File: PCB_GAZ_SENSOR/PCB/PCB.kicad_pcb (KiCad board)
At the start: 2 copper layers, 68.6 x 53.3 mm, 8 parts, among them P1 Power, P2 Analog, P3 Digital, P4 Digital, P5 CONN_01X01, P6 CONN_01X01, P7 CONN_01X01, P8 CONN_01X01

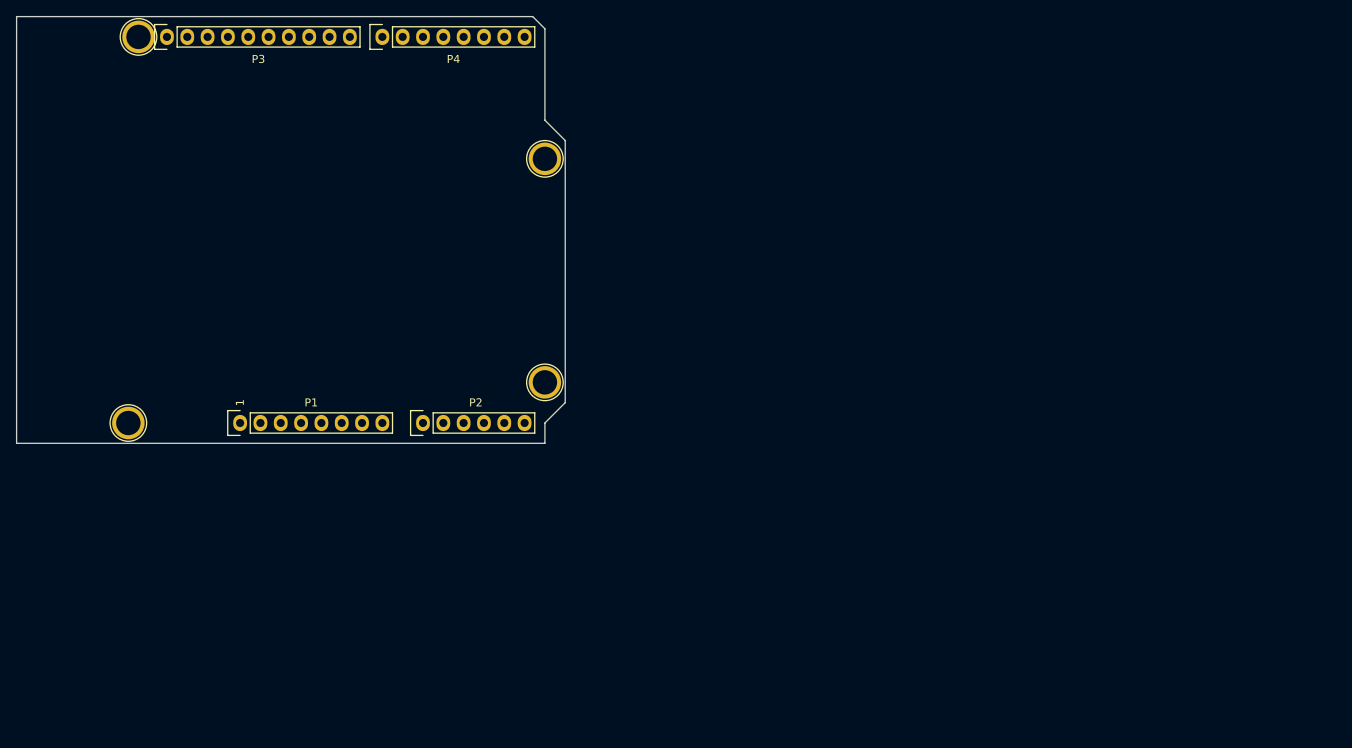
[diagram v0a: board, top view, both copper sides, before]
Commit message: final version
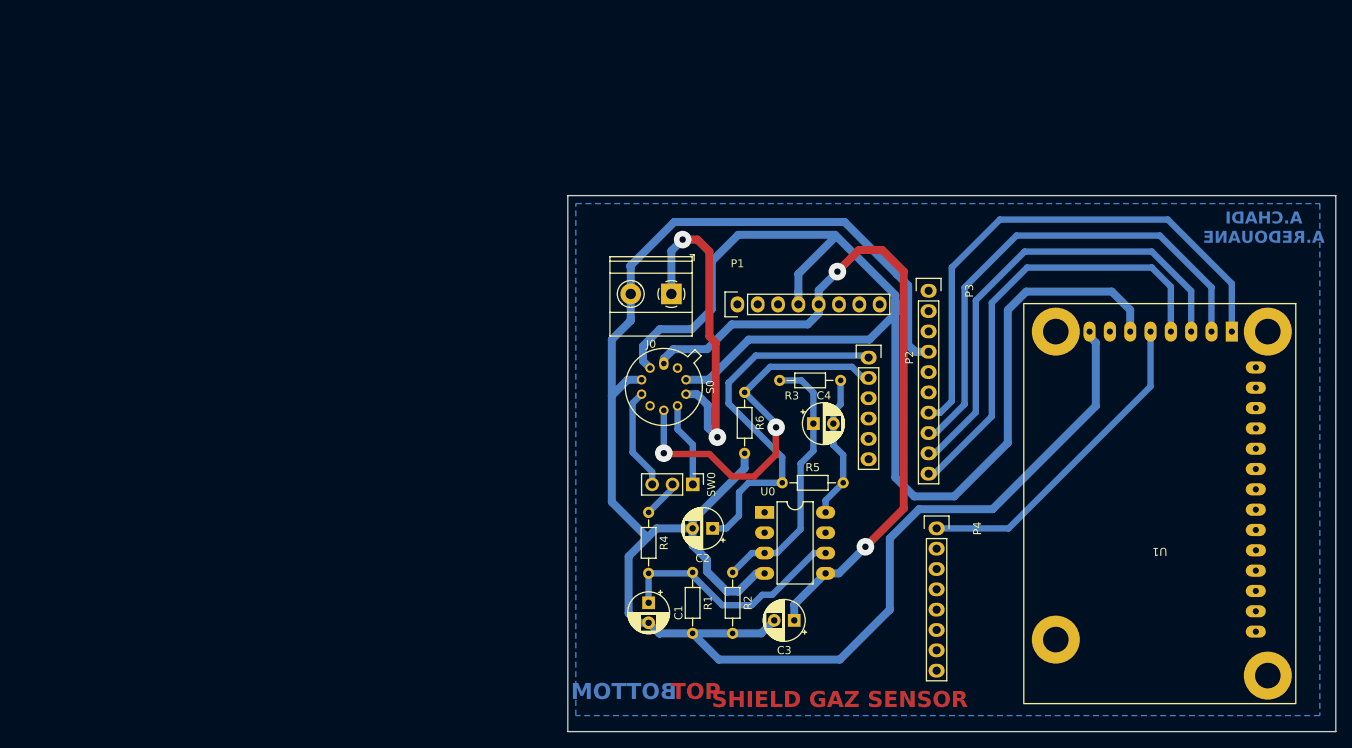
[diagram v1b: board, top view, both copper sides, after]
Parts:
- removed P5, P6, P7, P8: CONN_01X01, Socket_Arduino_Uno:Arduino_1pin
- added C1: 100n, Capacitor_THT:CP_Radial_D5.0mm_P2.50mm, F.Cu at (190.0, 146.3)
- added C2: 100n, Capacitor_THT:CP_Radial_D5.0mm_P2.50mm, F.Cu at (198.0, 137.0)
- added C3: 100n, Capacitor_THT:CP_Radial_D5.0mm_P2.50mm, F.Cu at (208.2, 148.5)
- added C4: 1u, Capacitor_THT:CP_Radial_D5.0mm_P2.50mm, F.Cu at (210.6, 123.9)
- added J0: Screw_Terminal_01x02, TerminalBlock_Phoenix:TerminalBlock_Phoenix_MKDS-1,5-2-5.08_1x02_P5.08mm_Horizontal, F.Cu at (192.8, 107.7)
- added R1: 100k, Resistor_THT:R_Axial_DIN0204_L3.6mm_D1.6mm_P7.62mm_Horizontal, F.Cu at (195.5, 142.5)
- added R2: R_CAL, Resistor_THT:R_Axial_DIN0204_L3.6mm_D1.6mm_P7.62mm_Horizontal, F.Cu at (200.5, 142.5)
- added R3: 100k, Resistor_THT:R_Axial_DIN0204_L3.6mm_D1.6mm_P7.62mm_Horizontal, F.Cu at (214.0, 118.5)
- added R4: 10k, Resistor_THT:R_Axial_DIN0204_L3.6mm_D1.6mm_P7.62mm_Horizontal, F.Cu at (190.0, 135.0)
- added R5: 1k, Resistor_THT:R_Axial_DIN0204_L3.6mm_D1.6mm_P7.62mm_Horizontal, F.Cu at (206.7, 131.3)
- added R6: R_adjust, Resistor_THT:R_Axial_DIN0204_L3.6mm_D1.6mm_P7.62mm_Horizontal, F.Cu at (202.0, 120.0)
- added S0: Sensor_Aime, Package_TO_SOT_THT:TO-5-10_Window, F.Cu at (191.9, 116.4)
- added SW0: SW_DPDT_x2, Connector_PinHeader_2.54mm:PinHeader_1x03_P2.54mm_Vertical, F.Cu at (195.5, 131.5)
- added U0: LTC1050, Package_DIP:DIP-8_W7.62mm_LongPads, F.Cu at (204.5, 135.0)
- added U1: RN2483_Breakout, mes_empreintes:RN2483_FOOTPRINT, F.Cu at (262.9, 112.4)
- moved P3 100.4 mm to (225.0, 107.3), turned to -90 degrees
- moved P4 92.6 mm to (226.0, 137.0), turned to -90 degrees
- moved P1 63.9 mm to (201.1, 109.0)
- moved P2 56.3 mm to (217.5, 115.7), turned to -90 degrees
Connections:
- P1 pad 1: Net-(P1-Pad1) -> unconnected-(P1-Pin_1)
- P1 pad 6: GND -> unconnected-(P1-Pin_6)
- P1 pad 7: GND -> unconnected-(P1-Pin_7)
- P2 pad 1: /A0 -> ADC_GAZ
- P2 pad 2: /A1 -> TempADC
- P3 pad 1: /A5(SCL) -> unconnected-(P3-Pin_1)
- P3 pad 2: /A4(SDA) -> unconnected-(P3-Pin_2)
- P3 pad 3: /AREF -> unconnected-(P3-Pin_3)
- P3 pad 7: /11(**/MOSI) -> /11(**/MOSI)
- P3 pad 8: /10(**/SS) -> /10(**/SS)
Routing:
- net GND: track 0.00 -> 236.2 mm
- net +3V3: track 0.00 -> 165.3 mm
- net +5V: track 0.00 -> 89.3 mm, vias 0 -> 2
- net /11(**/MOSI): track 0.00 -> 67.0 mm
- net /10(**/SS): track 0.00 -> 62.6 mm
- net /9(**): track 0.00 -> 58.6 mm
- net /8: track 0.00 -> 55.9 mm
- net TempADC: track 0.00 -> 48.5 mm, vias 0 -> 2
- net ADC_GAZ: track 0.00 -> 47.0 mm
- net +15V: track 0.00 -> 42.8 mm, vias 0 -> 2
- net /7: track 0.00 -> 40.9 mm
- net Net-(U0--): track 0.00 -> 33.3 mm
- net Net-(U0-+): track 0.00 -> 30.5 mm
- net Net-(C4-Pad2): track 0.00 -> 18.3 mm
- net Net-(S0-GazSensorRight): track 0.00 -> 12.8 mm
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- added copper zone on B.Cu, net GND
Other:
- board size 68.6 x 53.3 mm -> 96 x 67 mm
- board text added: "A.CHADI A.REDOUANE"
- board text added: "BOTTOM"
- board text added: "SHIELD GAZ SENSOR"
- board text added: "TOP"
- board text removed: "1"
